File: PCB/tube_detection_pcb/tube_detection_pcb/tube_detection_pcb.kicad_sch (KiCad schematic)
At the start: 12 parts, among them J1 B6B-XH-A, U1 DM3CQF1003L01, U2 DM3CQF1003L01, U3 DM3CQF1003L01, U4 DM3CQF1003L01, U5 DM3CQF1003L01, U6 SN74HC165N

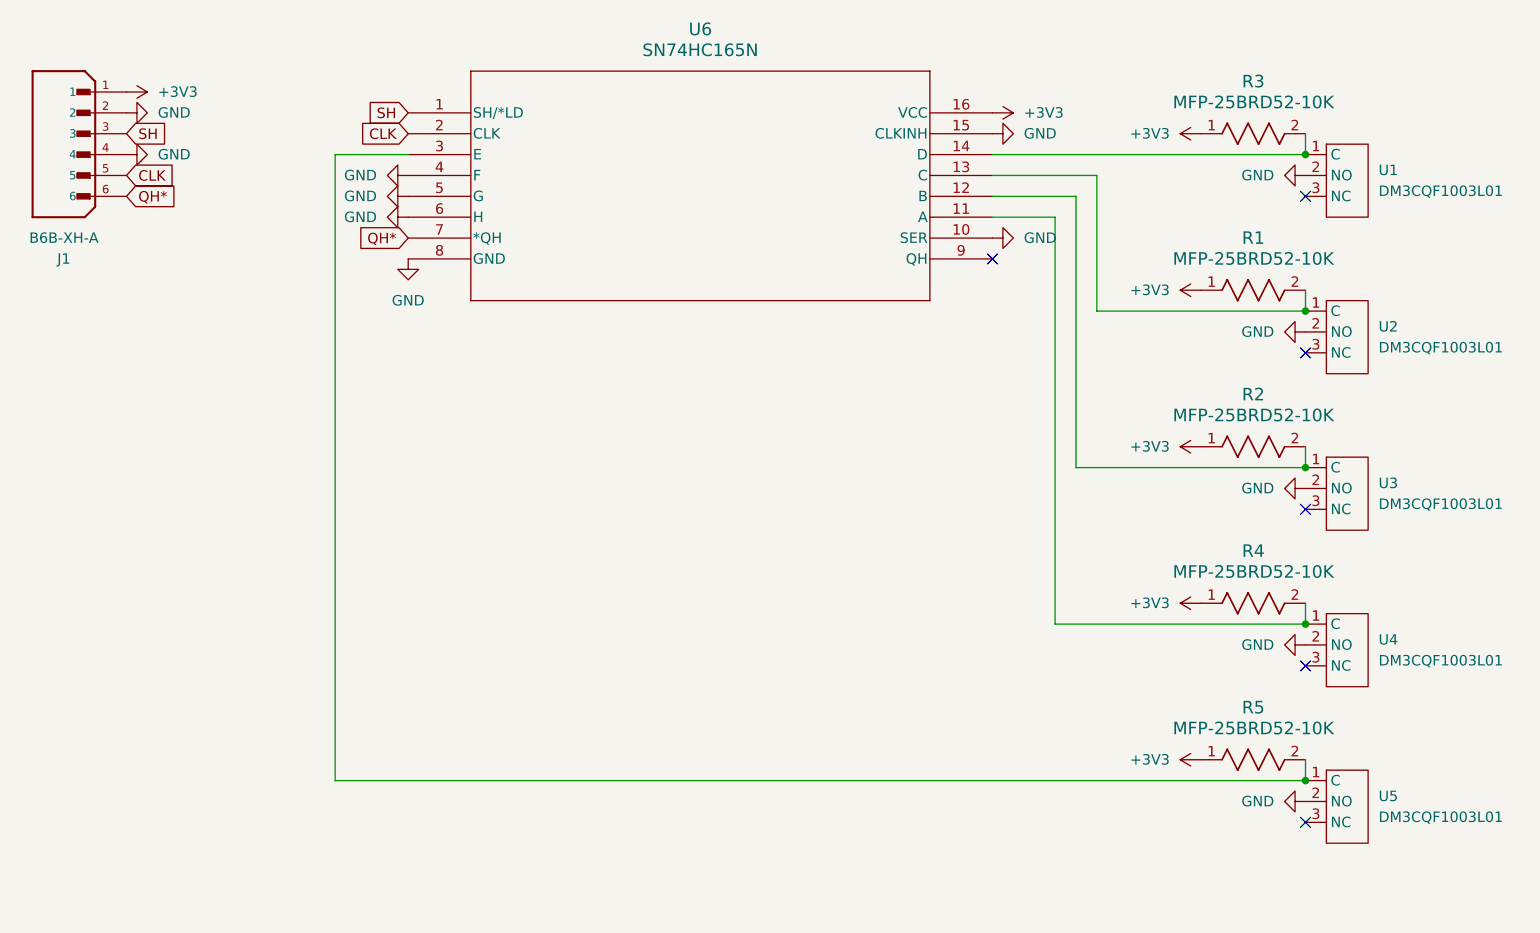
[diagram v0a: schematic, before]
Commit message: PCB updates
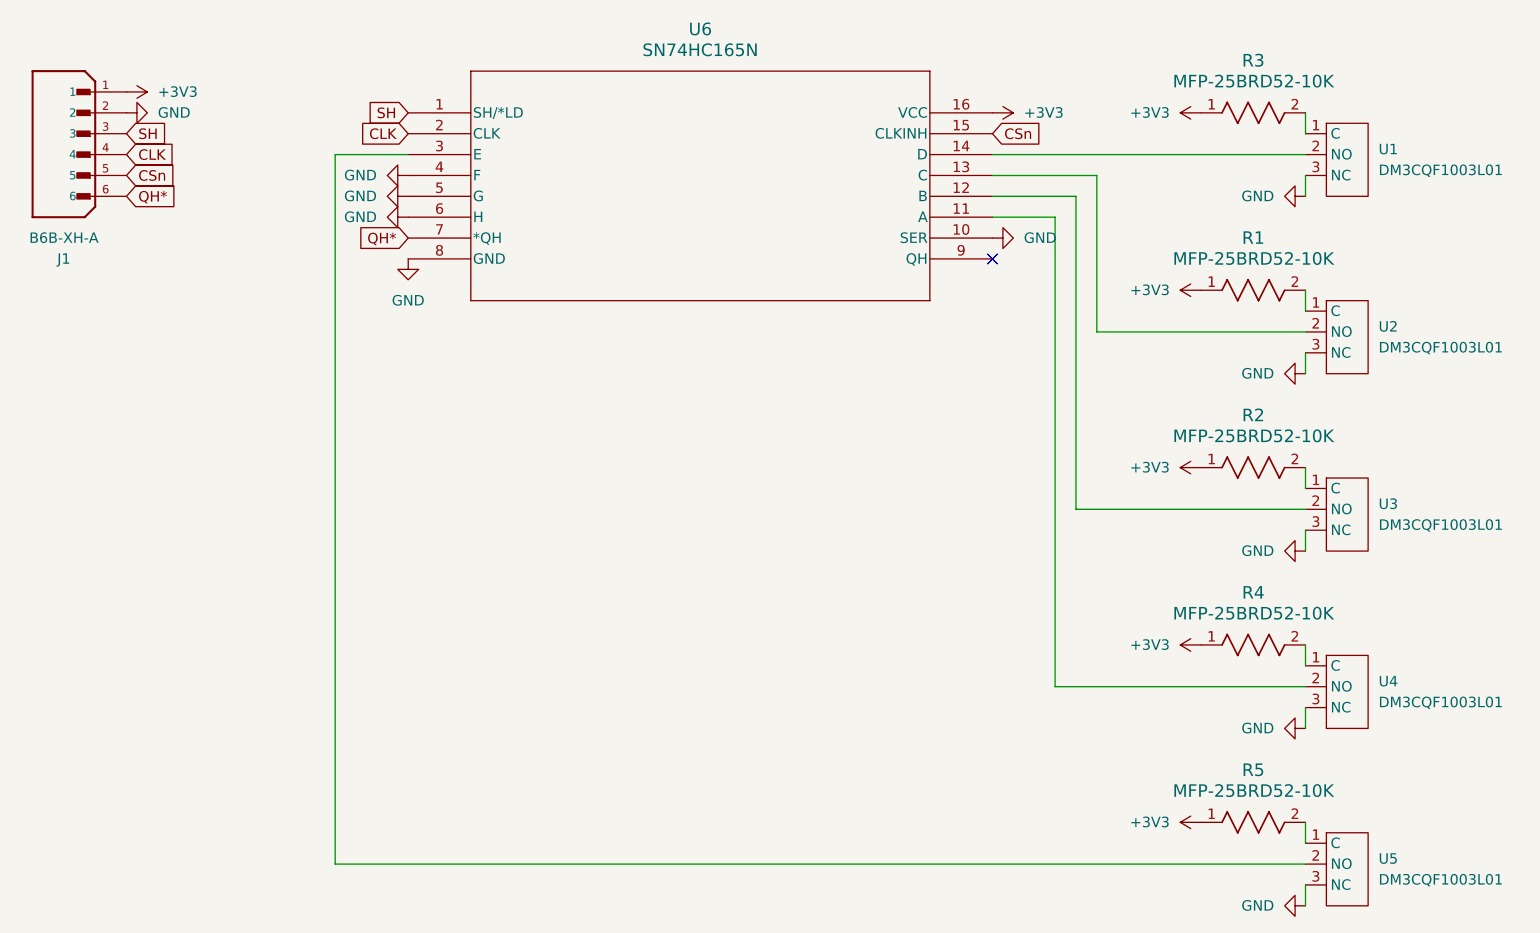
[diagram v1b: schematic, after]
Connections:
- net CLK: now also J1.4; no longer J1.5
- net GND: now also U1.3 (NC), U2.3 (NC), U3.3 (NC), U4.3 (NC), U5.3 (NC); no longer J1.4, U1.2 (NO), U2.2 (NO), U3.2 (NO), U4.2 (NO), U5.2 (NO), U6.15 (CLKINH)
- net at R1.2, U2.1 (C): no longer U6.13 (C)
- net at R5.2, U5.1 (C): no longer U6.3 (E)
- net at R3.2, U1.1 (C): no longer U6.14 (D)
- net at R4.2, U4.1 (C): no longer U6.11 (A)
- net at R2.2, U3.1 (C): no longer U6.12 (B)
- new net: U3.2 (NO), U6.12 (B)
- new net: U5.2 (NO), U6.3 (E)
- new net: U1.2 (NO), U6.14 (D)
- new net: U4.2 (NO), U6.11 (A)
- new net: U2.2 (NO), U6.13 (C)
- new net CSn: J1.5, U6.15 (CLKINH)
- no-connect marks 6 -> 1
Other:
- moved on the sheet: R3, U1

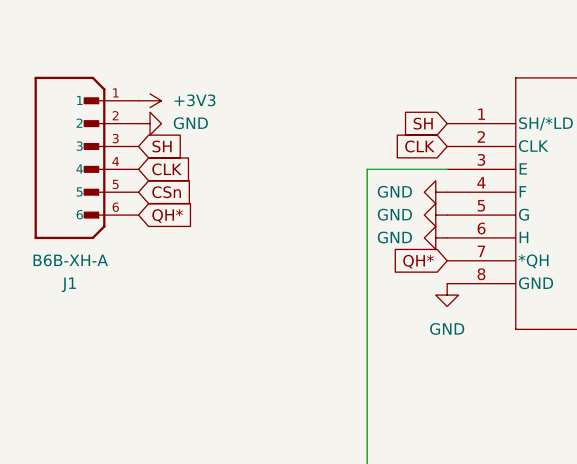
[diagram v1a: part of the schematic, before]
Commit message: pcb finishing touches
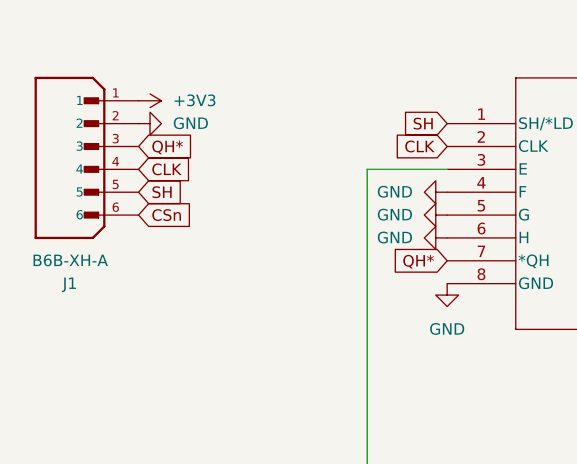
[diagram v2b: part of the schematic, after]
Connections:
- net CSn: now also J1.6; no longer J1.5
- net QH*: now also J1.3; no longer J1.6
- net SH: now also J1.5; no longer J1.3
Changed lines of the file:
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@@
 	(global_label "QH*"
 		(shape input)
-		(at 36.83 60.96 0)
+		(at 36.83 53.34 0)
 		(fields_autoplaced yes)
 		(effects
@@
 		)
 		(property "Intersheetrefs" "${INTERSHEET_REFS}"
-			(at 43.4438 60.96 0)
+			(at 43.4438 53.34 0)
 			(effects
 				(font
@@
 	(global_label "SH"
 		(shape input)
-		(at 36.83 53.34 0)
+		(at 36.83 58.42 0)
 		(fields_autoplaced yes)
 		(effects
@@
 		)
 		(property "Intersheetrefs" "${INTERSHEET_REFS}"
-			(at 42.3552 53.34 0)
+			(at 42.3552 58.42 0)
 			(effects
 				(font
@@
 	(global_label "CSn"
 		(shape input)
-		(at 36.83 58.42 0)
+		(at 36.83 60.96 0)
 		(fields_autoplaced yes)
 		(effects
@@
 		)
 		(property "Intersheetrefs" "${INTERSHEET_REFS}"
-			(at 43.4437 58.42 0)
+			(at 43.4437 60.96 0)
 			(effects
 				(font
